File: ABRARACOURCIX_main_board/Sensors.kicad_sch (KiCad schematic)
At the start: 21 parts, among them U1 STM32F429ZIT6, U2 ICM-42688-P

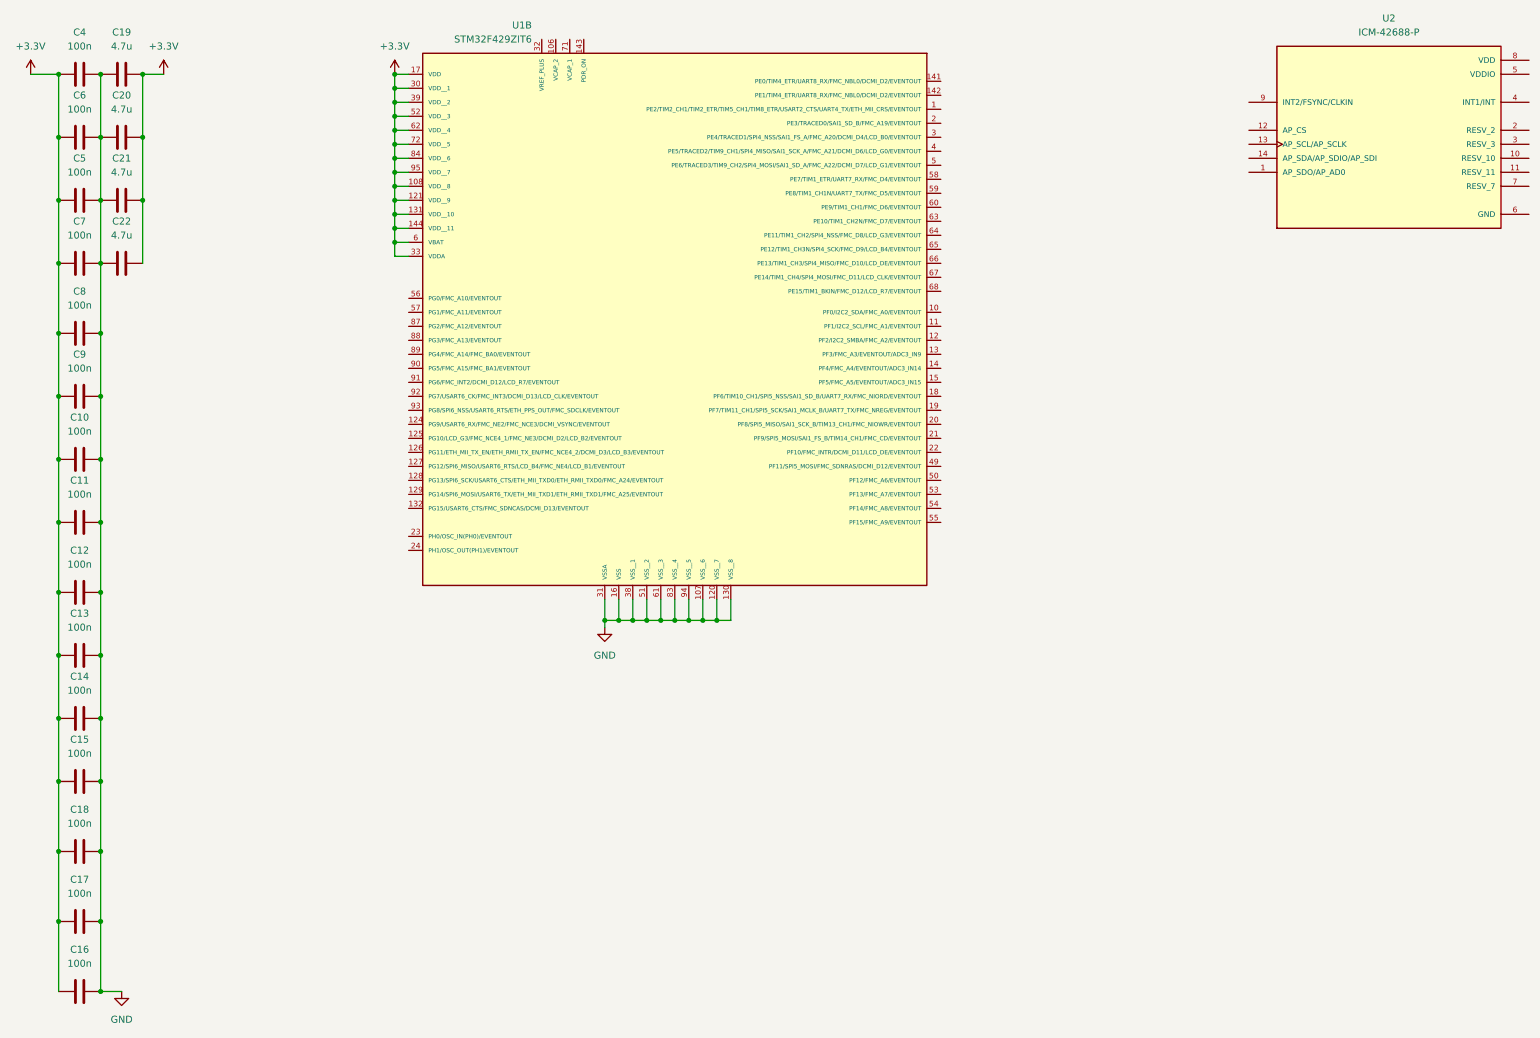
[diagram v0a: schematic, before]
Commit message: Commit de kicad
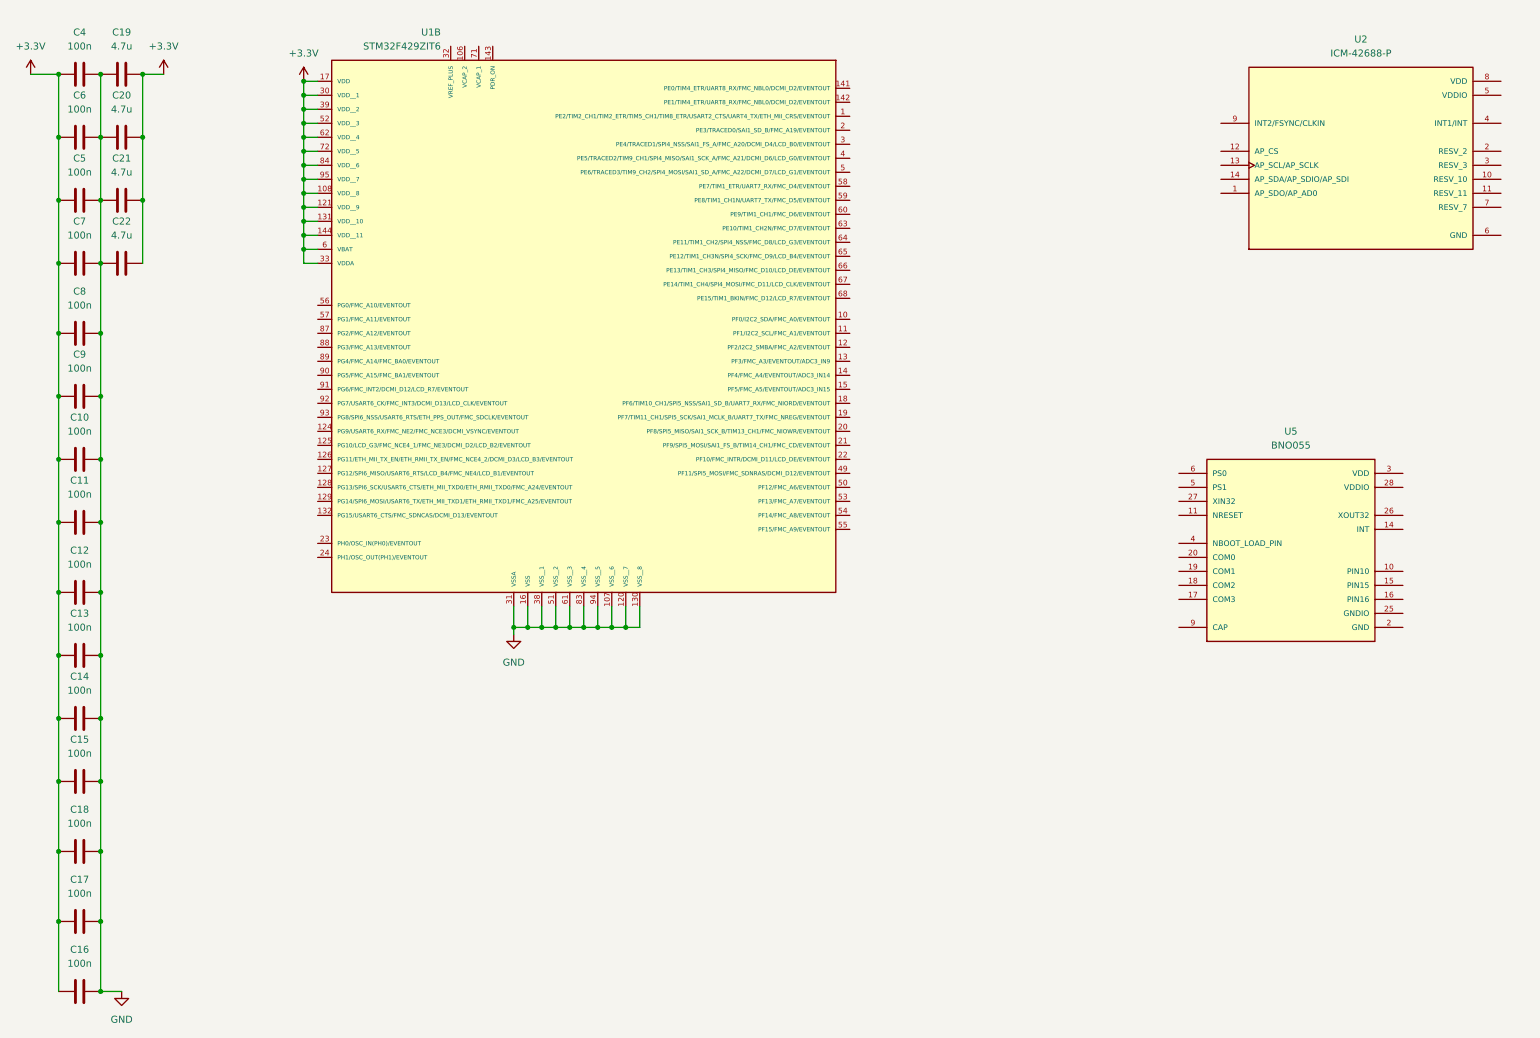
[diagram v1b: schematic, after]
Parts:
- added U5: BNO055, BNO055:LGA28R50P4X10_380X520X100, symbol GAUL_ABRARACOURCIX:BNO055
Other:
- moved on the sheet: U1B, U2
